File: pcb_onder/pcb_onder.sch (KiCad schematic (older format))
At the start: 18 parts

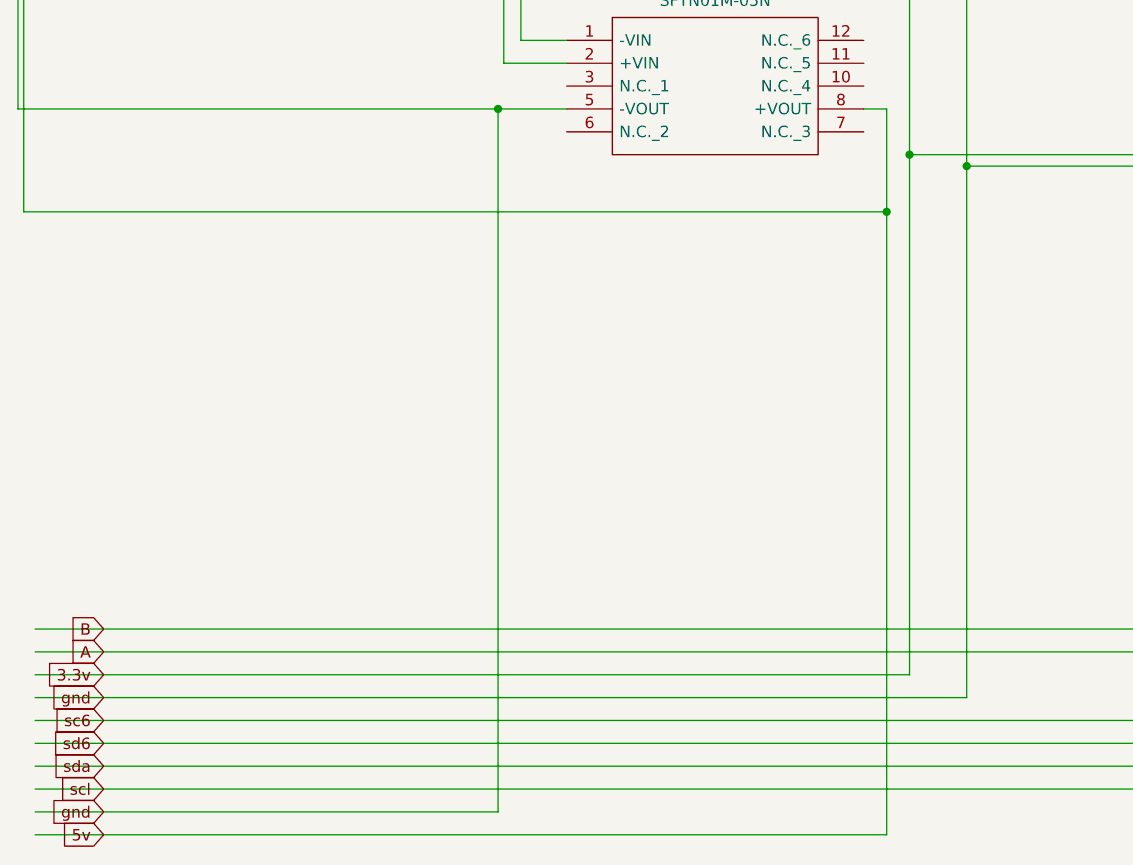
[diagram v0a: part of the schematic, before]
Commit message: pcb onder gemaakt
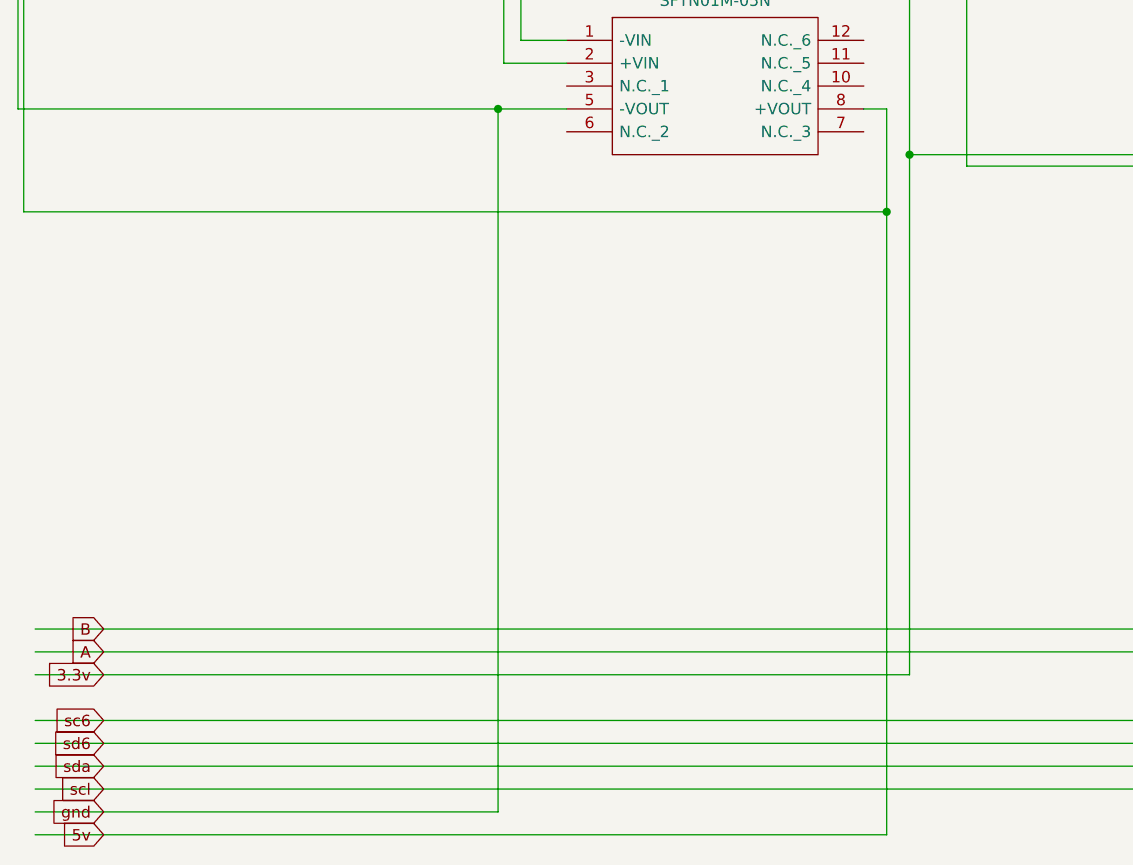
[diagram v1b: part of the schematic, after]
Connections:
- wire segments 232 -> 230
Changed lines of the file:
@@
 Wire Wire Line
 	950  11075 4675 11075
-Text GLabel 1250 10475 0    50   Input ~ 0
-gnd
 Text GLabel 1250 10375 0    50   Input ~ 0
 3.3v
@@
 Wire Wire Line
 	5025 7050 5025 7200
-Wire Wire Line
-	950  10475 5025 10475
 Wire Wire Line
 	4625 6850 4625 6250
@@
 Wire Wire Line
 	7100 8150 7100 7575
-Connection ~ 5025 8150
-Wire Wire Line
-	5025 8150 5025 10475
 Wire Wire Line
 	10075 4000 10075 6625

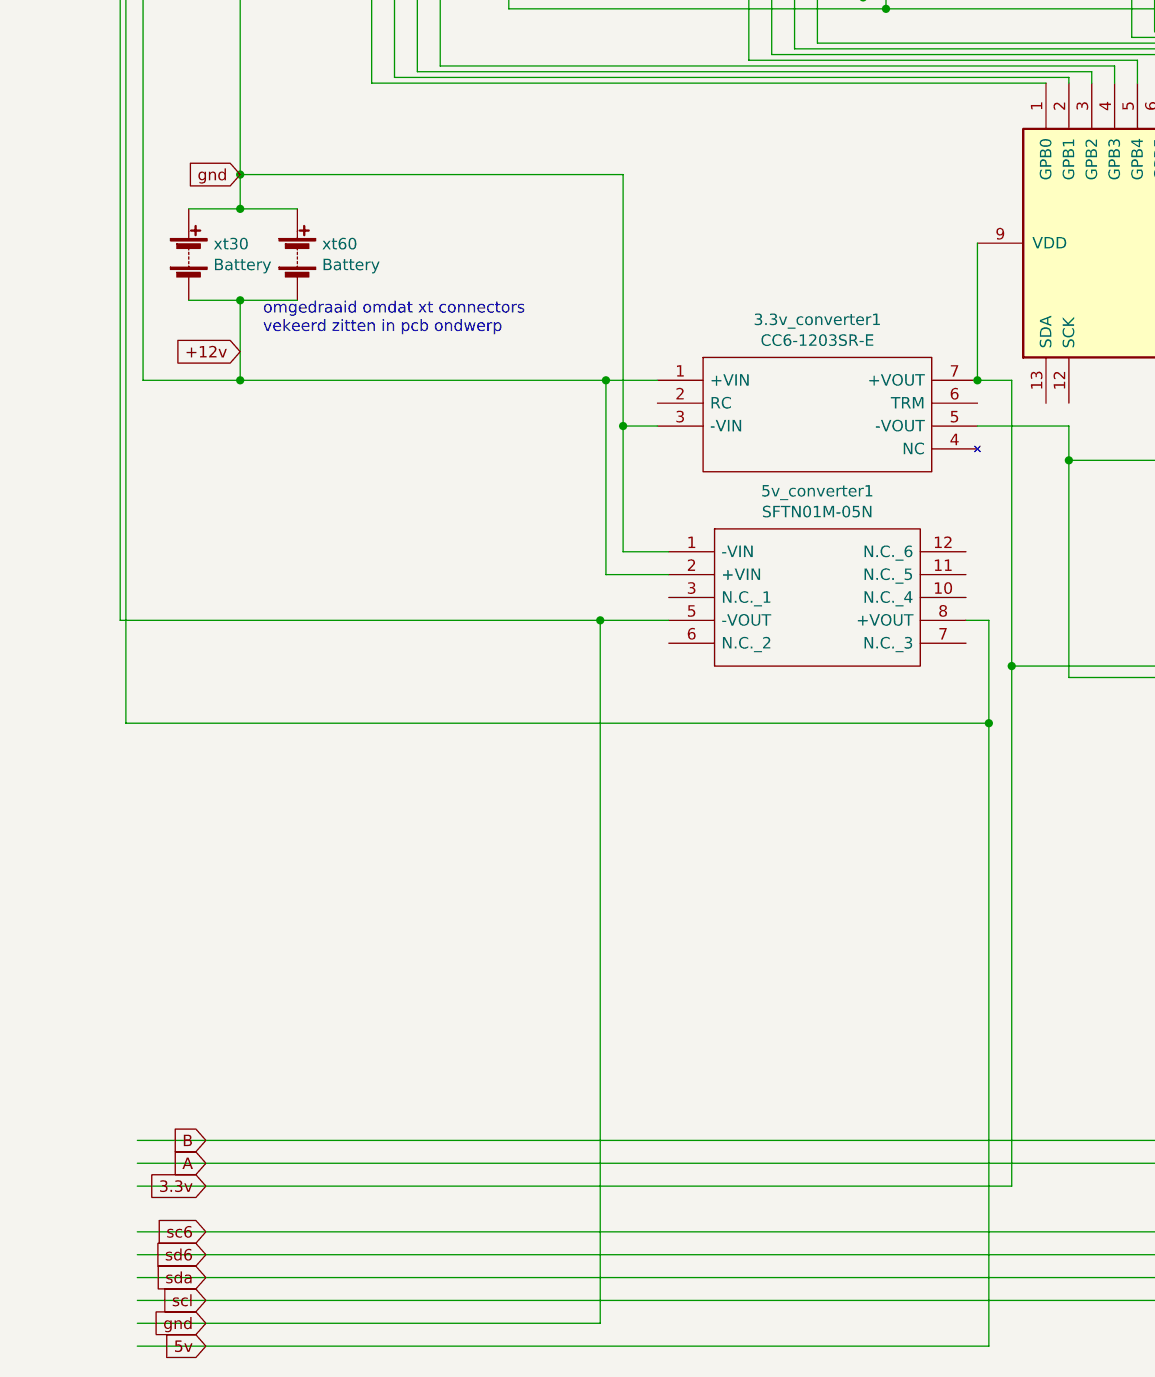
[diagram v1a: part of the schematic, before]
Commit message: pcb_onder y
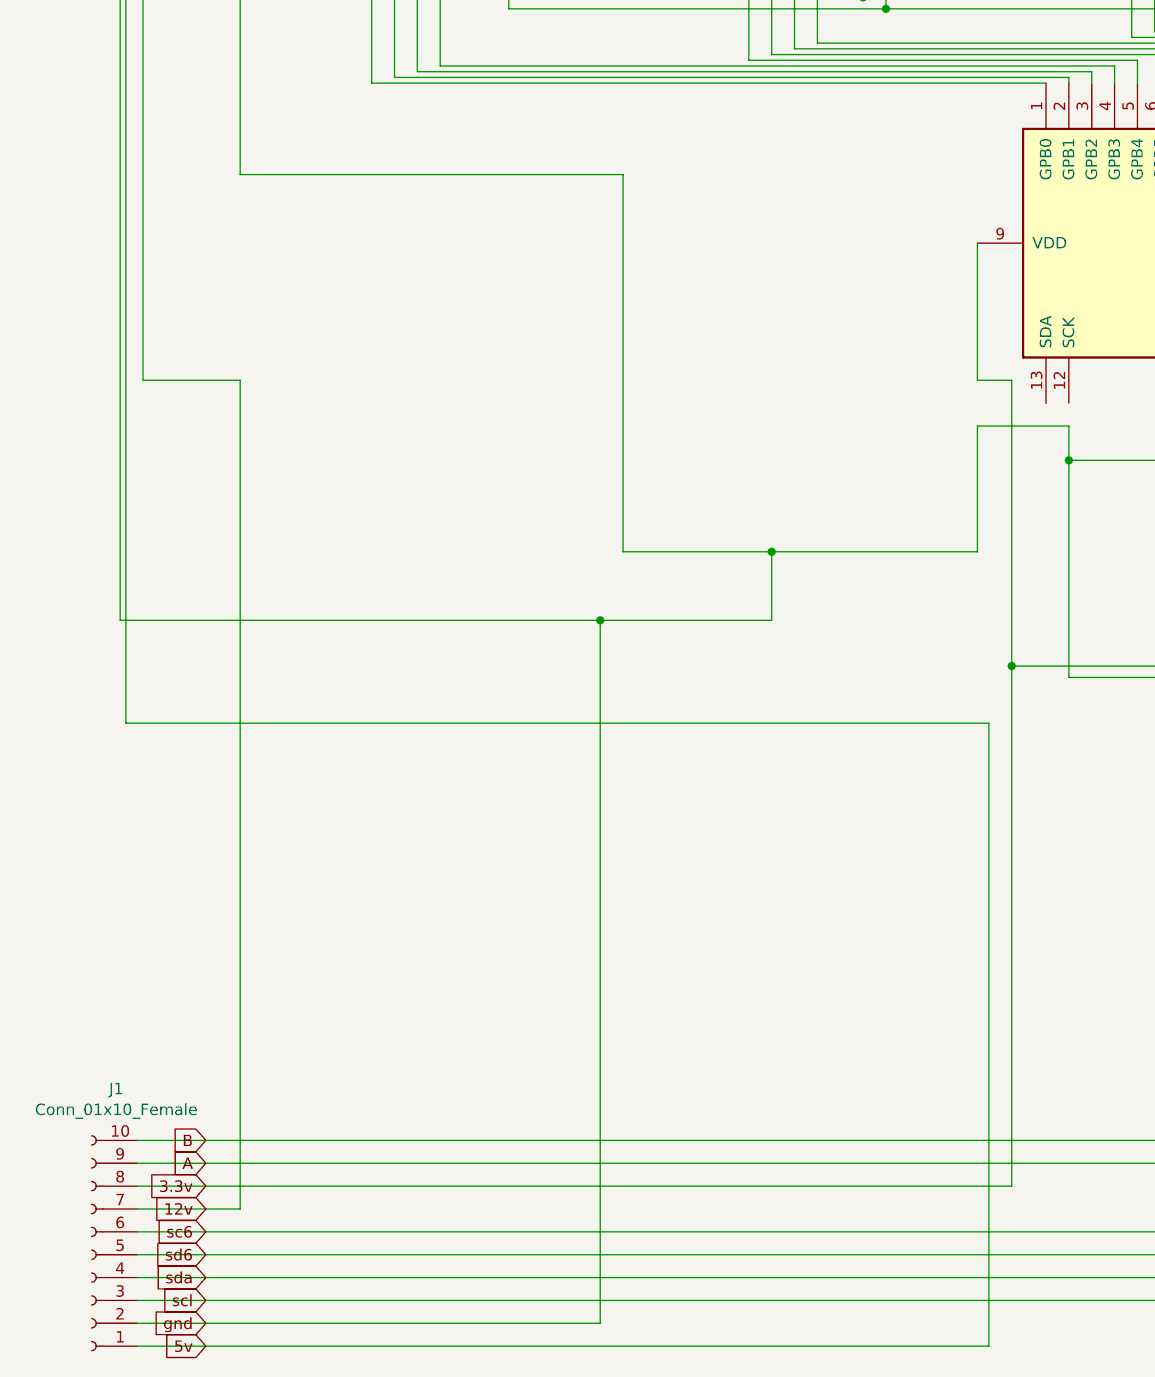
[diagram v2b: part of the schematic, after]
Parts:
- removed 3.3v_converter1: CC6-1203SR-E, custom:CC60512SRE, symbol cc6-1203sr-e:CC6-1203SR-E
- removed 5v_converter1: SFTN01M-05N, custom:SFTN01M05N, symbol sftn01m-05n:SFTN01M-05N
- removed xt30: Battery, Connector_AMASS:AMASS_XT30U-F_1x02_P5.0mm_Vertical, symbol Device:Battery
- removed xt60: Battery, Connector_AMASS:AMASS_XT60-F_1x02_P7.20mm_Vertical, symbol Device:Battery
- added J1: Conn_01x10_Female, custom:10x_conn, symbol Connector:Conn_01x10_Female
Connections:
- net labels added: 12v
- net labels removed: +12v
- wire segments 230 -> 221
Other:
- note removed: "omgedraaid omdat xt connectors \nvekeerd zitten in pcb ondwerp"
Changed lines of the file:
@@
 	5750 4050 5750 4150
 Connection ~ 4075 4050
-$Comp
-L Device:Battery xt30
-U 1 1 6636FCC1
-P 1175 6300
-F 0 "xt30" H 1283 6346 50  0000 L CNN
-F 1 "Battery" H 1283 6255 50  0000 L CNN
-F 2 "Connector_AMASS:AMASS_XT30U-F_1x02_P5.0mm_Vertical" V 1175 6360 50  0001 C CNN
-F 3 "~" V 1175 6360 50  0001 C CNN
-	1    1175 6300
-	1    0    0    -1
-$EndComp
-$Comp
-L Device:Battery xt60
-U 1 1 66371272
-P 1650 6300
-F 0 "xt60" H 1758 6346 50  0000 L CNN
-F 1 "Battery" H 1758 6255 50  0000 L CNN
-F 2 "Connector_AMASS:AMASS_XT60-F_1x02_P7.20mm_Vertical" V 1650 6360 50  0001 C CNN
-F 3 "~" V 1650 6360 50  0001 C CNN
-	1    1650 6300
-	1    0    0    -1
-$EndComp
-Wire Wire Line
-	1175 6100 1400 6100
-Wire Wire Line
-	1650 6500 1400 6500
-Connection ~ 1400 6100
-Wire Wire Line
-	1400 6100 1650 6100
-Wire Wire Line
-	1400 6500 1400 6850
-Connection ~ 1400 6500
-Wire Wire Line
-	1400 6500 1175 6500
-Text GLabel 1400 6725 0    50   Input ~ 0
-+12v
-Text GLabel 1400 5950 0    50   Input ~ 0
-gnd
-Text Notes 1500 6650 0    50   ~ 0
-omgedraaid omdat xt connectors \nvekeerd zitten in pcb ondwerp
 Wire Wire Line
 	1400 4125 2325 4125
@@
 	975  6850 1400 6850
 Connection ~ 2425 4050
-$Comp
-L cc6-1203sr-e:CC6-1203SR-E 3.3v_converter1
-U 1 1 66378F04
-P 3225 6850
-F 0 "3.3v_converter1" H 3925 7115 50  0000 C CNN
-F 1 "CC6-1203SR-E" H 3925 7024 50  0000 C CNN
-F 2 "custom:CC60512SRE" H 4475 6950 50  0001 L CNN
-F 3 "https://product.tdk.com/system/files/dam/doc/product/power/switching-power/dc-dc-converter/catalog/cc-e_e.pdf" H 4475 6850 50  0001 L CNN
-F 4 "DC-DC Converters, On-board type, Output: 3.96W, 3.3V, Isolated type, Option: SMD type" H 4475 6750 50  0001 L CNN "Description"
-F 5 "8.8" H 4475 6650 50  0001 L CNN "Height"
-F 6 "TDK" H 4475 6550 50  0001 L CNN "Manufacturer_Name"
-F 7 "CC6-1203SR-E" H 4475 6450 50  0001 L CNN "Manufacturer_Part_Number"
-F 8 "967-CC6-1203SR-E" H 4475 6350 50  0001 L CNN "Mouser Part Number"
-F 9 "https://www.mouser.co.uk/ProductDetail/TDK-Lambda/CC6-1203SR-E?qs=Vwh6e7toGLi4J%2FzloL2n3g%3D%3D" H 4475 6250 50  0001 L CNN "Mouser Price/Stock"
-F 10 "CC6-1203SR-E" H 4475 6150 50  0001 L CNN "Arrow Part Number"
-F 11 "https://www.arrow.com/en/products/cc6-1203sr-e/tdk-lambda-americas?region=nac" H 4475 6050 50  0001 L CNN "Arrow Price/Stock"
-	1    3225 6850
-	1    0    0    -1
-$EndComp
-$Comp
-L sftn01m-05n:SFTN01M-05N 5v_converter1
-U 1 1 66379F5D
-P 3275 7600
-F 0 "5v_converter1" H 3925 7865 50  0000 C CNN
-F 1 "SFTN01M-05N" H 3925 7774 50  0000 C CNN
-F 2 "custom:SFTN01M05N" H 4425 7700 50  0001 L CNN
-F 3 "https://www.meanwell.com/webapp/product/search.aspx?prod=SFTN01-N" H 4425 7600 50  0001 L CNN
-F 4 "Isolated DC/DC Converters - SMD 1W 12Vin 5Vout 20-200mA SMT Unregulated" H 4425 7500 50  0001 L CNN "Description"
-F 5 "7.6" H 4425 7400 50  0001 L CNN "Height"
-F 6 "Mean Well" H 4425 7300 50  0001 L CNN "Manufacturer_Name"
-F 7 "SFTN01M-05N" H 4425 7200 50  0001 L CNN "Manufacturer_Part_Number"
-F 8 "709-SFTN01M-05N" H 4425 7100 50  0001 L CNN "Mouser Part Number"
-F 9 "https://www.mouser.co.uk/ProductDetail/MEAN-WELL/SFTN01M-05N?qs=A6eO%252BMLsxmQLvWwJN5Fn%252BQ%3D%3D" H 4425 7000 50  0001 L CNN "Mouser Price/Stock"
-	1    3275 7600
-	1    0    0    -1
-$EndComp
-Wire Wire Line
-	1400 6850 3000 6850
-Wire Wire Line
-	3000 6850 3000 7700
-Wire Wire Line
-	3000 7700 3275 7700
-Connection ~ 1400 6850
-Wire Wire Line
-	3000 6850 3225 6850
-Connection ~ 3000 6850
-Wire Wire Line
-	3275 7600 3075 7600
-Wire Wire Line
-	3075 7600 3075 7050
-Wire Wire Line
-	3075 7050 3225 7050
-Wire Wire Line
-	3075 7050 3075 5950
 Wire Wire Line
 	3075 5950 1400 5950
-Connection ~ 3075 7050
-Connection ~ 1400 5950
-Wire Wire Line
-	1400 5950 1400 6100
 $Comp
 L tcs3472_color_sensor:tcs3472_color_sensor kleur_sensor_1
@@
 scl
 Wire Wire Line
-	3275 7900 2975 7900
-Wire Wire Line
 	2975 7900 2975 10975
 Wire Wire Line
@@
 	4675 11075 4675 8350
 Wire Wire Line
-	4675 7900 4575 7900
-Wire Wire Line
 	950  11075 4675 11075
 Text GLabel 1250 10375 0    50   Input ~ 0
@@
 Wire Wire Line
 	4775 6850 4775 8100
-Connection ~ 4625 6850
 Wire Wire Line
 	1975 5150 1975 5550
@@
 	900  8350 4675 8350
 Connection ~ 1975 3025
-Connection ~ 4675 8350
-Wire Wire Line
-	4675 8350 4675 7900
+Text GLabel 1250 10475 0    50   Input ~ 0
+12v
+$Comp
+L Connector:Conn_01x10_Female J1
+U 1 1 66673A65
+P 750 10675
+F 0 "J1" H 642 9950 50  0000 C CNN
+F 1 "Conn_01x10_Female" H 642 10041 50  0000 C CNN
+F 2 "custom:10x_conn" H 750 10675 50  0001 C CNN
+F 3 "~" H 750 10675 50  0001 C CNN
+	1    750  10675
+	-1   0    0    1
+$EndComp
+Wire Wire Line
+	1400 10475 1400 6850
+Wire Wire Line
+	950  10475 1400 10475
+Wire Wire Line
+	3725 7900 3725 7600
+Wire Wire Line
+	3075 7600 3725 7600
+Wire Wire Line
+	2975 7900 3725 7900
+Wire Wire Line
+	3725 7600 4625 7600
+Wire Wire Line
+	4625 7600 4625 7050
+Connection ~ 3725 7600
+Wire Wire Line
+	3075 5950 3075 7600
 $EndSCHEMATC
